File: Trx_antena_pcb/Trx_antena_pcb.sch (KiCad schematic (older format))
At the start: 3 parts

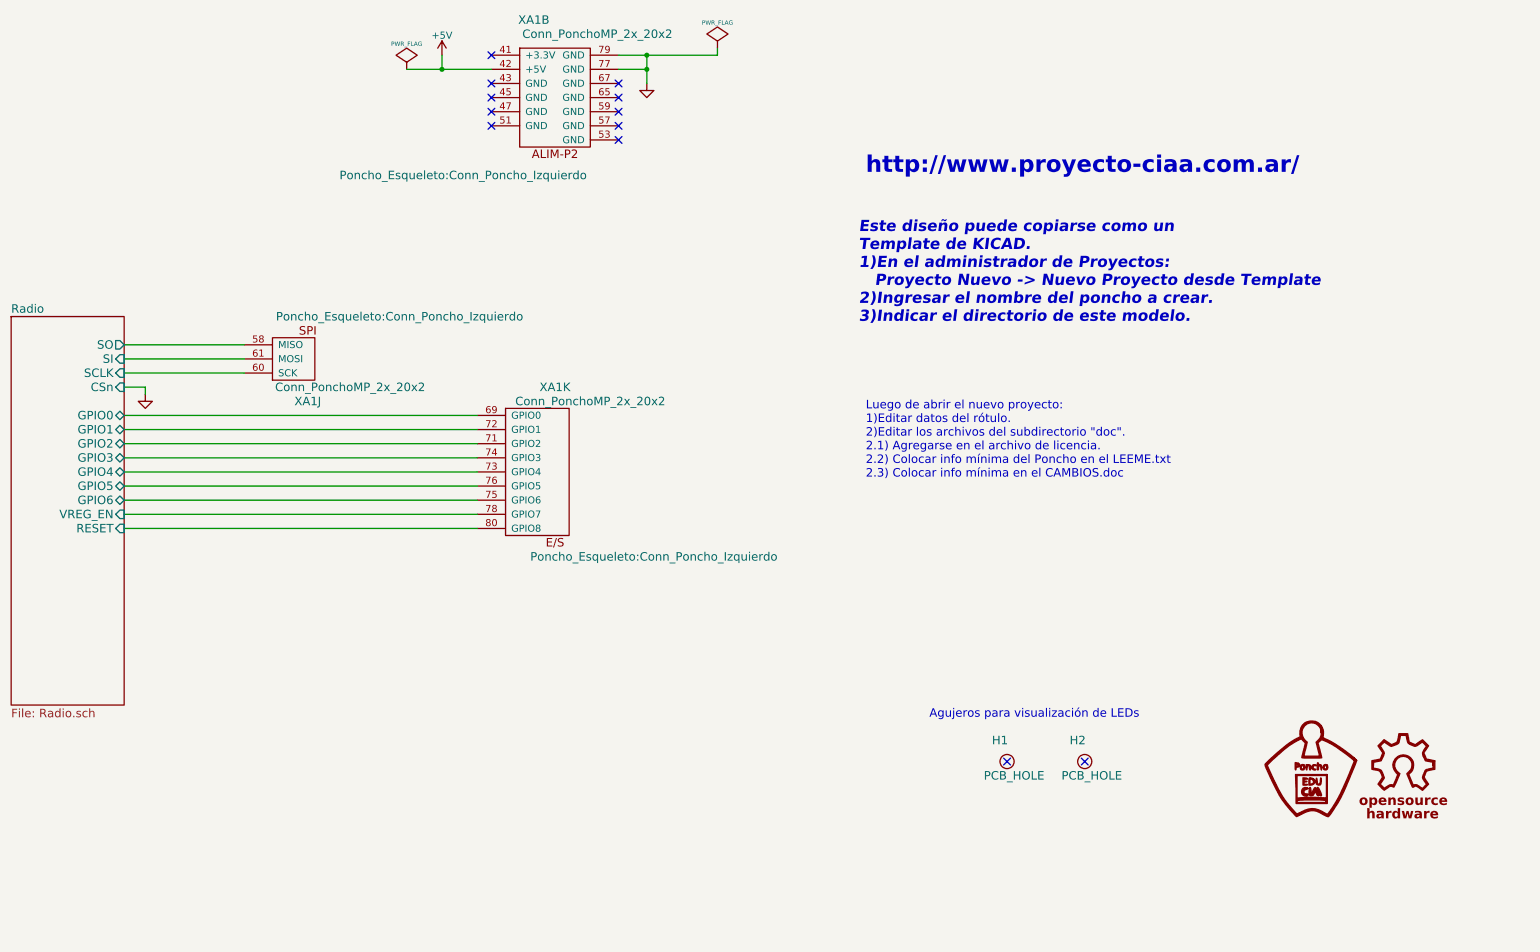
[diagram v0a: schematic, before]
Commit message: cuarta correccion: revision2 en /doc
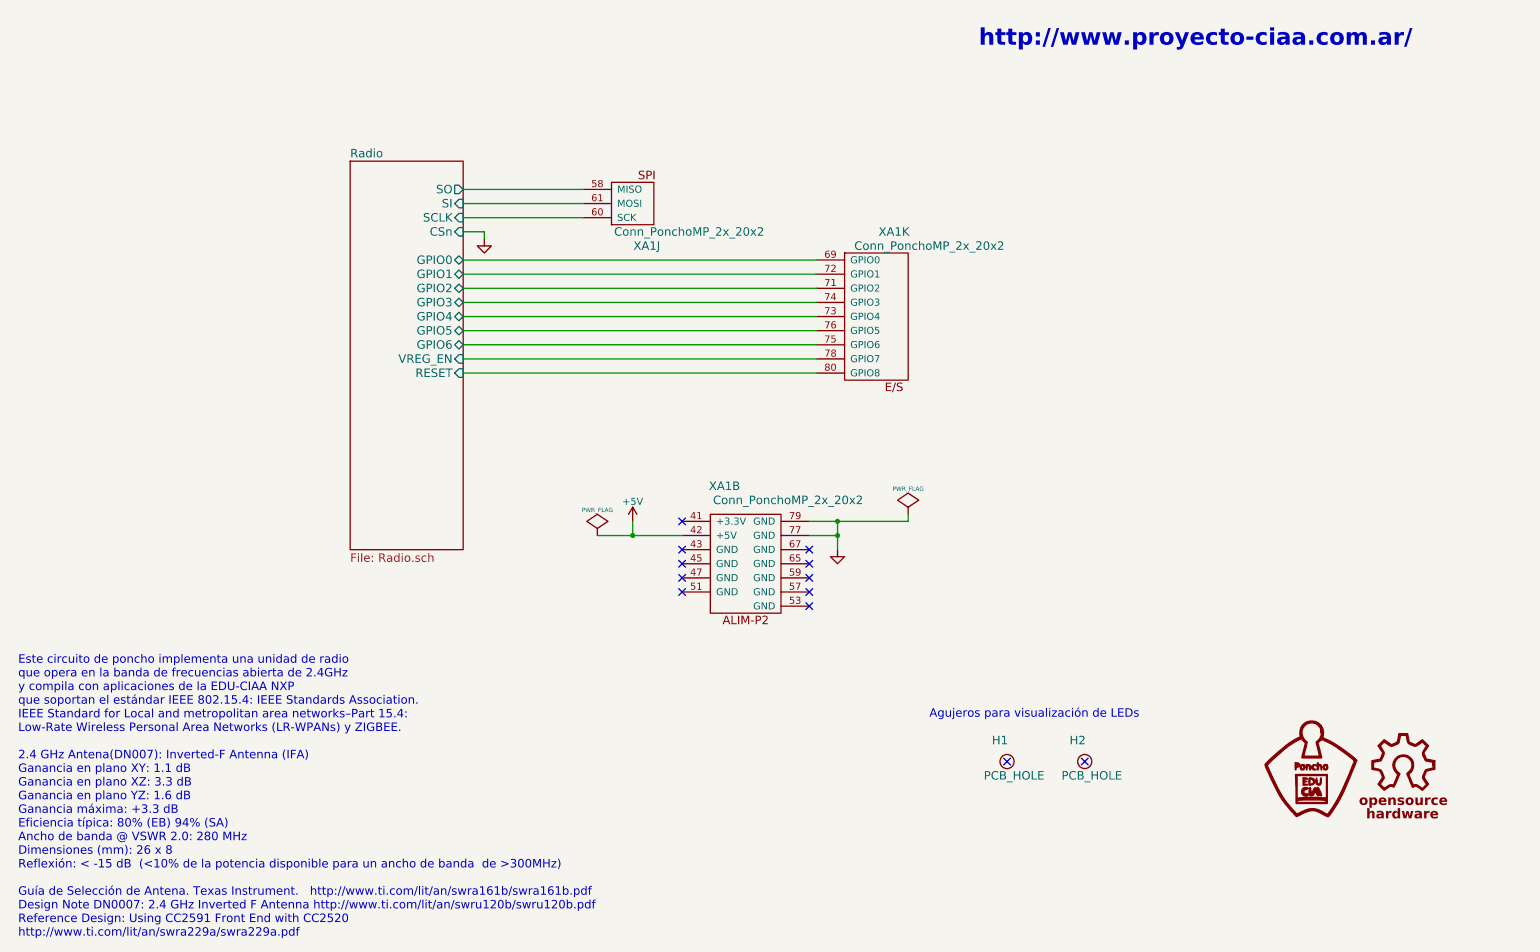
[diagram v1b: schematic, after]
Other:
- note added: "Este circuito de poncho implementa una unidad de radio \nque opera en la banda de frecuencias abierta de 2.4GHz \ny compila con aplicaciones de la EDU-CIAA NXP \nque soportan el estándar IEEE 802.15.4: IEEE Standards Association. \nIEEE Standard for Local and metropolitan area networks–Part 15.4: \nLow-Rate Wireless Personal Area Networks (LR-WPANs) y ZIGBEE.\n\n2.4 GHz Antena(DN007): Inverted-F 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"
- note removed: "Este diseño puede copiarse como un \nTemplate de KICAD. \n1)En el administrador de Proyectos: \n Proyecto Nuevo -> Nuevo Proyecto desde Template\n2)Ingresar el nombre del poncho a crear.\n3)Indicar el directorio de este modelo."
- note removed: "Luego de abrir el nuevo proyecto:\n1)Editar datos del rótulo.\n2)Editar los archivos del subdirectorio "doc".\n2.1) Agregarse en el archivo de licencia.\n2.2) Colocar info mínima del Poncho en el LEEME.txt\n2.3) Colocar info mínima en el CAMBIOS.doc"
- moved on the sheet: XA1B, XA1J, XA1K
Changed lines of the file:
@@
 EESchema Schematic File Version 2
-LIBS:device
+LIBS:power
 LIBS:Trx_antena_pcb-cache
 EELAYER 25 0
@@
 Comment1 "https://github.com/ciaa/Ponchos/tree/master/modelos/doc"
 Comment2 "Basado en el template de Diego Brengi - UNLaM"
-Comment3 "Autor y Licencia del poncho (Juan Vicente Montilla-FIUBA). Ver directorio \"doc\""
-Comment4 "https://github.com/Juanvmont/Poncho-EDU-CIAA-NXP-RF-2.4GHz-Antena-PCB.git"
+Comment3 "Revisor designado (Esp. Ing. Patricio Bos-FIUBA)."
+Comment4 "Autor y Licencia del poncho (Esp. Ing. Juan Vicente Montilla-FIUBA). Ver directorio \"doc\""
 $EndDescr
 $Comp
@@
 	1    0    0    -1
 $EndComp
-Text Notes 6950 2850 0    79   Italic 16
-Este diseño puede copiarse como un \nTemplate de KICAD. \n1)En el administrador de Proyectos:  \n   Proyecto Nuevo -> Nuevo Proyecto desde Template\n2)Ingresar el nombre del poncho a crear.\n3)Indicar el directorio de este modelo.
-Text Notes 7000 1800 0    118  ~ 24
+Text Notes 7800 900  0    118  ~ 24
 http://www.proyecto-ciaa.com.ar/
 $Comp
 L Conn_PonchoMP_2x_20x2 XA1
 U 11 1 560E5596
-P 4700 3800
-F 0 "XA1" H 4600 4300 60  0000 C CNN
-F 1 "Conn_PonchoMP_2x_20x2" H 4350 4200 60  0000 C CNN
-F 2 "Poncho_Esqueleto:Conn_Poncho_Izquierdo" H 3900 3100 60  0000 C CNN
-F 3 "" H 4550 4150 60  0000 C CNN
-	11   4700 3800
+P 7100 2700
+F 0 "XA1" H 7000 3200 60  0000 C CNN
+F 1 "Conn_PonchoMP_2x_20x2" H 6750 3100 60  0000 C CNN
+F 2 "Poncho_Esqueleto:Conn_Poncho_Izquierdo" H 6300 2000 60  0001 C CNN
+F 3 "" H 6950 3050 60  0000 C CNN
+	11   7100 2700
 	-1   0    0    -1
 $EndComp
-Text Notes 7000 3950 0    60   ~ 0
-Luego de abrir el nuevo proyecto:\n1)Editar datos del rótulo.\n2)Editar los archivos del subdirectorio "doc".\n2.1) Agregarse en el archivo de licencia.\n2.2) Colocar info mínima del Poncho en el LEEME.txt\n2.3) Colocar info mínima en el CAMBIOS.doc
 $Comp
 L Conn_PonchoMP_2x_20x2 XA1
 U 10 1 560E54EF
-P 2950 3100
-F 0 "XA1" H 2850 3400 60  0000 C CNN
-F 1 "Conn_PonchoMP_2x_20x2" H 2550 3300 60  0000 C CNN
-F 2 "Poncho_Esqueleto:Conn_Poncho_Izquierdo" H 2200 2800 60  0000 C CNN
-F 3 "" H 2800 3450 60  0000 C CNN
-	10   2950 3100
+P 5350 2000
+F 0 "XA1" H 5250 2300 60  0000 C CNN
+F 1 "Conn_PonchoMP_2x_20x2" H 4950 2200 60  0000 C CNN
+F 2 "Poncho_Esqueleto:Conn_Poncho_Izquierdo" H 4600 1700 60  0001 C CNN
+F 3 "" H 5200 2350 60  0000 C CNN
+	10   5350 2000
 	-1   0    0    1
 $EndComp
@@
 L PWR_FLAG #FLG01
 U 1 1 560EE826
-P 3750 1050
-F 0 "#FLG01" H 3750 1145 30  0001 C CNN
-F 1 "PWR_FLAG" H 3750 1230 30  0000 C CNN
-F 2 "" H 3750 1050 60  0000 C CNN
-F 3 "" H 3750 1050 60  0000 C CNN
-	1    3750 1050
+P 5100 4350
+F 0 "#FLG01" H 5100 4445 30  0001 C CNN
+F 1 "PWR_FLAG" H 5100 4530 30  0000 C CNN
+F 2 "" H 5100 4350 60  0000 C CNN
+F 3 "" H 5100 4350 60  0000 C CNN
+	1    5100 4350
 	1    0    0    -1
 $EndComp
@@
 L GND #PWR02
 U 1 1 560EE345
-P 5450 1150
-F 0 "#PWR02" H 5450 1150 30  0001 C CNN
-F 1 "GND" H 5450 1080 30  0001 C CNN
-F 2 "" H 5450 1150 60  0000 C CNN
-F 3 "" H 5450 1150 60  0000 C CNN
-	1    5450 1150
-	1    0    0    -1
-$EndComp
-NoConn ~ 5250 1150
-NoConn ~ 5250 1250
-NoConn ~ 5250 1350
-NoConn ~ 5250 1450
-NoConn ~ 5250 1550
-NoConn ~ 4350 1450
-NoConn ~ 4350 950
+P 6800 4450
+F 0 "#PWR02" H 6800 4450 30  0001 C CNN
+F 1 "GND" H 6800 4380 30  0001 C CNN
+F 2 "" H 6800 4450 60  0000 C CNN
+F 3 "" H 6800 4450 60  0000 C CNN
+	1    6800 4450
+	1    0    0    -1
+$EndComp
+NoConn ~ 6600 4450
+NoConn ~ 6600 4550
+NoConn ~ 6600 4650
+NoConn ~ 6600 4750
+NoConn ~ 6600 4850
+NoConn ~ 5700 4750
+NoConn ~ 5700 4250
 $Comp
 L Conn_PonchoMP_2x_20x2 XA1
 U 2 1 560EE110
-P 4800 1250
-F 0 "XA1" H 4650 1800 60  0000 C CNN
-F 1 "Conn_PonchoMP_2x_20x2" H 5100 1700 60  0000 C CNN
-F 2 "Poncho_Esqueleto:Conn_Poncho_Izquierdo" H 4150 700 60  0000 C CNN
-F 3 "" H 4650 1600 60  0000 C CNN
-	2    4800 1250
+P 6150 4550
+F 0 "XA1" H 6000 5100 60  0000 C CNN
+F 1 "Conn_PonchoMP_2x_20x2" H 6450 5000 60  0000 C CNN
+F 2 "Poncho_Esqueleto:Conn_Poncho_Izquierdo" H 5500 4000 60  0001 C CNN
+F 3 "" H 6000 4900 60  0000 C CNN
+	2    6150 4550
 	1    0    0    -1
 $EndComp
@@
 L PWR_FLAG #FLG03
 U 1 1 560EDE73
-P 5950 900
-F 0 "#FLG03" H 5950 995 30  0001 C CNN
-F 1 "PWR_FLAG" H 5950 1080 30  0000 C CNN
-F 2 "" H 5950 900 60  0000 C CNN
-F 3 "" H 5950 900 60  0000 C CNN
-	1    5950 900
-	1    0    0    -1
-$EndComp
-NoConn ~ 4350 1350
-NoConn ~ 4350 1250
-NoConn ~ 4350 1150
+P 7300 4200
+F 0 "#FLG03" H 7300 4295 30  0001 C CNN
+F 1 "PWR_FLAG" H 7300 4380 30  0000 C CNN
+F 2 "" H 7300 4200 60  0000 C CNN
+F 3 "" H 7300 4200 60  0000 C CNN
+	1    7300 4200
+	1    0    0    -1
+$EndComp
+NoConn ~ 5700 4650
+NoConn ~ 5700 4550
+NoConn ~ 5700 4450
 $Comp
 L PCB_HOLE H2
@@
 Text Notes 7450 5650 0    60   ~ 0
 Agujeros para visualización de LEDs
-Connection ~ 4000 1050
-Wire Wire Line
-	4000 1050 4000 950
-Wire Wire Line
-	3750 1050 4350 1050
-Connection ~ 5450 1050
-Wire Wire Line
-	5250 950  5950 950
-Wire Wire Line
-	5450 950  5450 1150
-Wire Wire Line
-	5250 1050 5450 1050
-Wire Wire Line
-	5950 950  5950 900
-Connection ~ 5450 950
-Wire Wire Line
-	2600 3000 1750 3000
-Wire Wire Line
-	2600 3100 1750 3100
-Wire Wire Line
-	2600 3200 1750 3200
-Wire Wire Line
-	1750 3500 4250 3500
-Wire Wire Line
-	4250 3600 1750 3600
-Wire Wire Line
-	1750 3700 4250 3700
-Wire Wire Line
-	1750 3800 4250 3800
-Wire Wire Line
-	1750 3900 4250 3900
-Wire Wire Line
-	1750 4000 4250 4000
-Wire Wire Line
-	1750 4100 4250 4100
+Connection ~ 5350 4350
+Wire Wire Line
+	5350 4350 5350 4250
+Wire Wire Line
+	5100 4350 5700 4350
+Connection ~ 6800 4350
+Wire Wire Line
+	6600 4250 7300 4250
+Wire Wire Line
+	6800 4250 6800 4450
+Wire Wire Line
+	6600 4350 6800 4350
+Wire Wire Line
+	7300 4250 7300 4200
+Connection ~ 6800 4250
+Wire Wire Line
+	5000 1900 4150 1900
+Wire Wire Line
+	5000 2000 4150 2000
+Wire Wire Line
+	5000 2100 4150 2100
+Wire Wire Line
+	4150 2400 6650 2400
+Wire Wire Line
+	6650 2500 4150 2500
+Wire Wire Line
+	4150 2600 6650 2600
+Wire Wire Line
+	4150 2700 6650 2700
+Wire Wire Line
+	4150 2800 6650 2800
+Wire Wire Line
+	4150 2900 6650 2900
+Wire Wire Line
+	4150 3000 6650 3000
 $Sheet
-S 950  2800 800  2750
+S 3350 1700 800  2750
 U 582F8126
 F0 "Radio" 60
 F1 "Radio.sch" 60
-F2 "SO" O R 1750 3000 60
-F3 "SI" I R 1750 3100 60
-F4 "VREG_EN" I R 1750 4200 60
-F5 "SCLK" I R 1750 3200 60
-F6 "GPIO0" B R 1750 3500 60
-F7 "GPIO1" B R 1750 3600 60
-F8 "GPIO2" B R 1750 3700 60
-F9 "GPIO3" B R 1750 3800 60
-F10 "GPIO4" B R 1750 3900 60
-F11 "GPIO5" B R 1750 4000 60
-F12 "CSn" I R 1750 3300 60
-F13 "GPIO6" B R 1750 4100 60
-F14 "RESET" I R 1750 4300 60
+F2 "SO" O R 4150 1900 60
+F3 "SI" I R 4150 2000 60
+F4 "VREG_EN" I R 4150 3100 60
+F5 "SCLK" I R 4150 2100 60
+F6 "GPIO0" B R 4150 2400 60
+F7 "GPIO1" B R 4150 2500 60
+F8 "GPIO2" B R 4150 2600 60
+F9 "GPIO3" B R 4150 2700 60
+F10 "GPIO4" B R 4150 2800 60
+F11 "GPIO5" B R 4150 2900 60
+F12 "CSn" I R 4150 2200 60
+F13 "GPIO6" B R 4150 3000 60
+F14 "RESET" I R 4150 3200 60
 $EndSheet
 Wire Wire Line
-	4250 4200 1750 4200
+	6650 3100 4150 3100
 $Comp
 L +5V #PWR04
 U 1 1 5851A27B
-P 4000 950
-F 0 "#PWR04" H 4000 800 50  0001 C CNN
-F 1 "+5V" H 4000 1090 50  0000 C CNN
-F 2 "" H 4000 950 50  0000 C CNN
-F 3 "" H 4000 950 50  0000 C CNN
-	1    4000 950
-	1    0    0    -1
-$EndComp
-Wire Wire Line
-	4250 4300 1750 4300
+P 5350 4250
+F 0 "#PWR04" H 5350 4100 50  0001 C CNN
+F 1 "+5V" H 5350 4390 50  0000 C CNN
+F 2 "" H 5350 4250 50  0000 C CNN
+F 3 "" H 5350 4250 50  0000 C CNN
+	1    5350 4250
+	1    0    0    -1
+$EndComp
+Wire Wire Line
+	6650 3200 4150 3200
 $Comp
 L GND #PWR05
 U 1 1 5852BF25
-P 1900 3350
-F 0 "#PWR05" H 1900 3350 30  0001 C CNN
-F 1 "GND" H 1900 3280 30  0001 C CNN
-F 2 "" H 1900 3350 60  0000 C CNN
-F 3 "" H 1900 3350 60  0000 C CNN
-	1    1900 3350
-	1    0    0    -1
-$EndComp
-Wire Wire Line
-	1900 3350 1900 3300
-Wire Wire Line
-	1900 3300 1750 3300
+P 4300 2250
+F 0 "#PWR05" H 4300 2250 30  0001 C CNN
+F 1 "GND" H 4300 2180 30  0001 C CNN
+F 2 "" H 4300 2250 60  0000 C CNN
+F 3 "" H 4300 2250 60  0000 C CNN
+	1    4300 2250
+	1    0    0    -1
+$EndComp
+Wire Wire Line
+	4300 2250 4300 2200
+Wire Wire Line
+	4300 2200 4150 2200
+Text Notes 1000 7200 0    60   ~ 0
+Este circuito de poncho implementa una unidad de radio \nque opera en la banda de frecuencias abierta de 2.4GHz \ny compila con aplicaciones de la EDU-CIAA NXP \nque soportan el estándar IEEE 802.15.4: IEEE Standards Association. \nIEEE Standard for Local and metropolitan area networks–Part 15.4: \nLow-Rate Wireless Personal Area Networks (LR-WPANs) y ZIGBEE.\n\n2.4 GHz Antena(DN007): Inverted-F Antenna (IFA) \nGanancia en plano XY: 1.1 dB\nGanancia en plano XZ: 3.3 dB\nGanancia en plano YZ: 1.6 dB\nGanancia máxima: +3.3 dB\nEficiencia típica: 80% (EB) 94% (SA)\nAncho de banda @ VSWR 2.0: 280 MHz\nDimensiones (mm): 26 x 8\nReflexión: < -15 dB  (<10% de la potencia disponible para un ancho de banda  de >300MHz)\n\nGuía de Selección de Antena. Texas Instrument.   http://www.ti.com/lit/an/swra161b/swra161b.pdf\nDesign Note DN0007: 2.4 GHz Inverted F Antenna http://www.ti.com/lit/an/swru120b/swru120b.pdf\nReference Design: Using CC2591 Front End with CC2520\nhttp://www.ti.com/lit/an/swra229a/swra229a.pdf
 $EndSCHEMATC
